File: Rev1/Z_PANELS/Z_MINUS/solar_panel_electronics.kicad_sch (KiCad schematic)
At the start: 24 parts, among them IC2 SM141K08TFV, IC3 SM141K04TFV, IC4 SM141K04TFV, IC5 SM141K04TFV, IC6 SM141K08TFV, U2 LTC3130EUDC-1-PBF

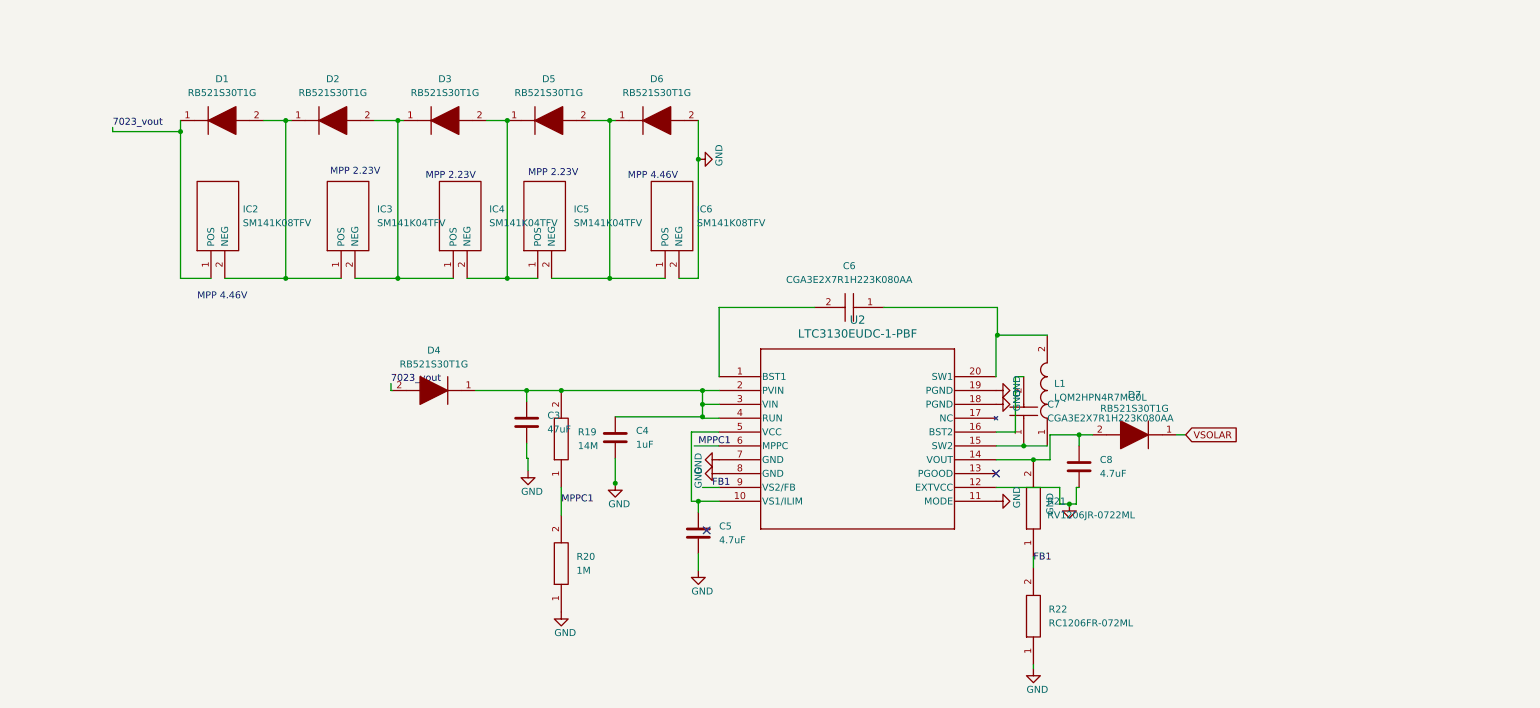
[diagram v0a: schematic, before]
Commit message: updated boards
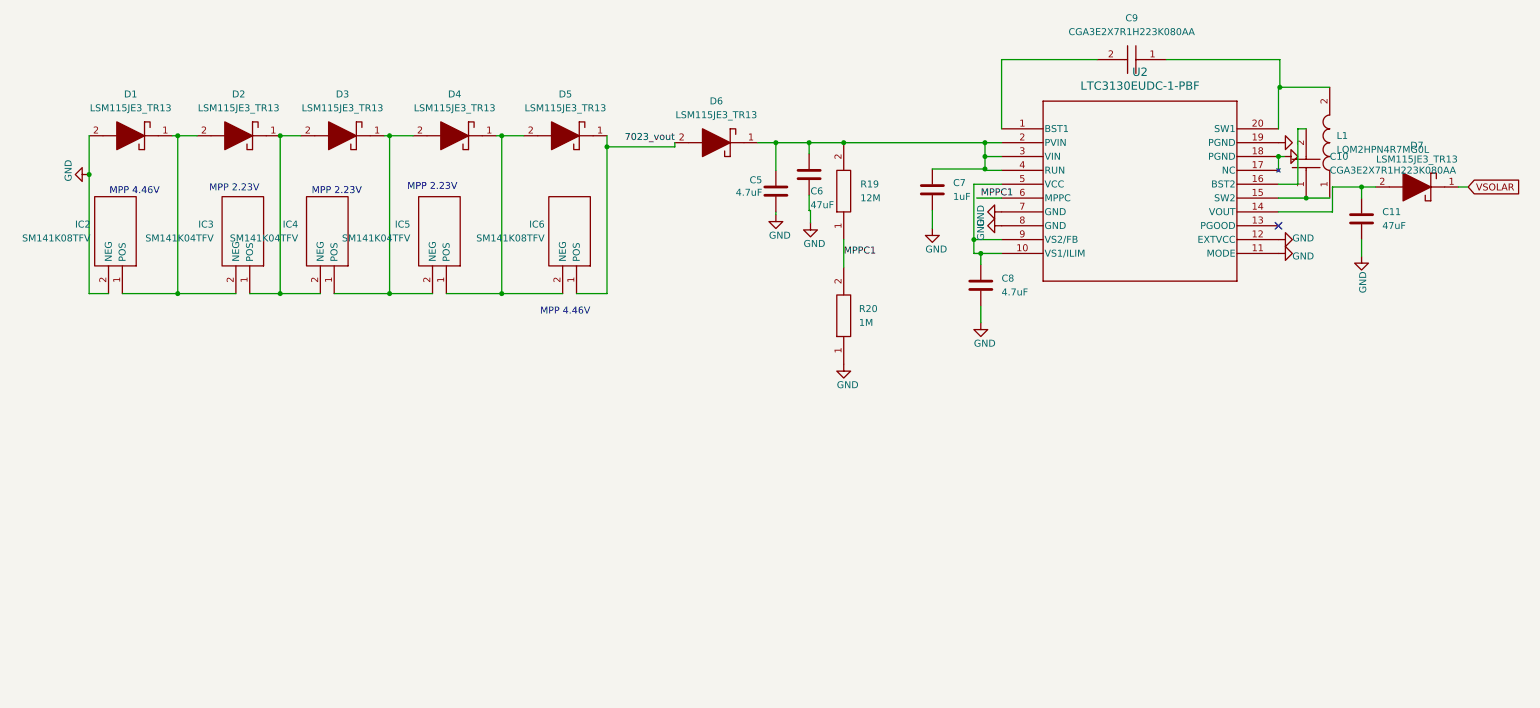
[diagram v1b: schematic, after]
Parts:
- removed C3: 47uF, Capacitor_SMD:C_0805_2012Metric, symbol PCM_Capacitor_AKL:C_0805
- removed C4: 1uF, Capacitor_SMD:C_0805_2012Metric, symbol PCM_Capacitor_AKL:C_0805
- removed C6, C7: CGA3E2X7R1H223K080AA, CAPC1608X90N, symbol AA_AUTO_LOADER:CGA3E2X7R1H223K080AA
- removed D1, D2, D3, D4, D5, D6, D7: RB521S30T1G, SODFL1608X70N, symbol AA_AUTO_LOADER:RB521S30T1G
- removed R21: RV1206JR-0722ML, RESC3116X65N, symbol AA_AUTO_LOADER:RV1206JR-0722ML
- removed R22: RC1206FR-072ML, RESC3116X65N, symbol AA_AUTO_LOADER:RC1206FR-072ML
- added C10, C9: CGA3E2X7R1H223K080AA, CAPC1608X90N, symbol AA_AUTO_LOADER:CGA3E2X7R1H223K080AA
- added C11, C6: 47uF, Capacitor_SMD:C_0805_2012Metric, symbol PCM_Capacitor_AKL:C_0805
- added C7: 1uF, Capacitor_SMD:C_0805_2012Metric, symbol PCM_Capacitor_AKL:C_0805
- added D1, D2, D3, D4, D5, D6, D7: LSM115JE3_TR13, DIOM5436X330N, symbol AA_AUTO_LOADER:LSM115JE3_TR13
- R19: value 14M -> 12M
- renumbered IC6 to IC2, IC5 to IC3, IC3 to IC5, IC2 to IC6
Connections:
- net FB1 is gone; now on an unnamed net: U2.9 (VS2/FB)
- net 7023_vout: now also D5.1, D6.2
- net GND: now also U2.17 (NC), C11.2, C6.2, C7.2, D1.2
- net VSOLAR: now also D7.1
- net at IC4.1 (POS), IC5.2 (NEG): now also D3.1, D4.2
- net at IC3.1 (POS), IC4.2 (NEG): now also D2.1, D3.2
- net at IC2.1 (POS), IC3.2 (NEG): now also D1.1, D2.2
- net at L1.1, U2.15 (SW2): now also C10.1
- net at L1.2, U2.20 (SW1): now also C9.1
- net at C8.1: now also U2.10 (VS1/ILIM), U2.5 (VCC); no longer U2.14 (VOUT)
- net at IC5.1 (POS), IC6.2 (NEG): now also D4.1, D5.2
- net at U2.1 (BST1): now also C9.2
- net at R19.2, U2.2 (PVIN), U2.3 (VIN)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: now also C5.1, C6.1, C7.1, D6.1
- net at U2.16 (BST2): now also C10.2
- new net: C11.1, D7.2, U2.14 (VOUT)
- no-connect marks 2 -> 1
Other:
- moved on the sheet: IC2, IC3, IC4, IC5, IC6
